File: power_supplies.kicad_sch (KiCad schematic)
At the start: 45 parts, among them IC4 MCP1792T-5002H_CB, IC5 MCP1792T-5002H_CB, J3 12V supply, J5 490107670612, Q3 2N7002BK,215, Q4 Si2333DS, Q5 2N7002BK,215, T1 760390014, U1 PIC10F322-IOT

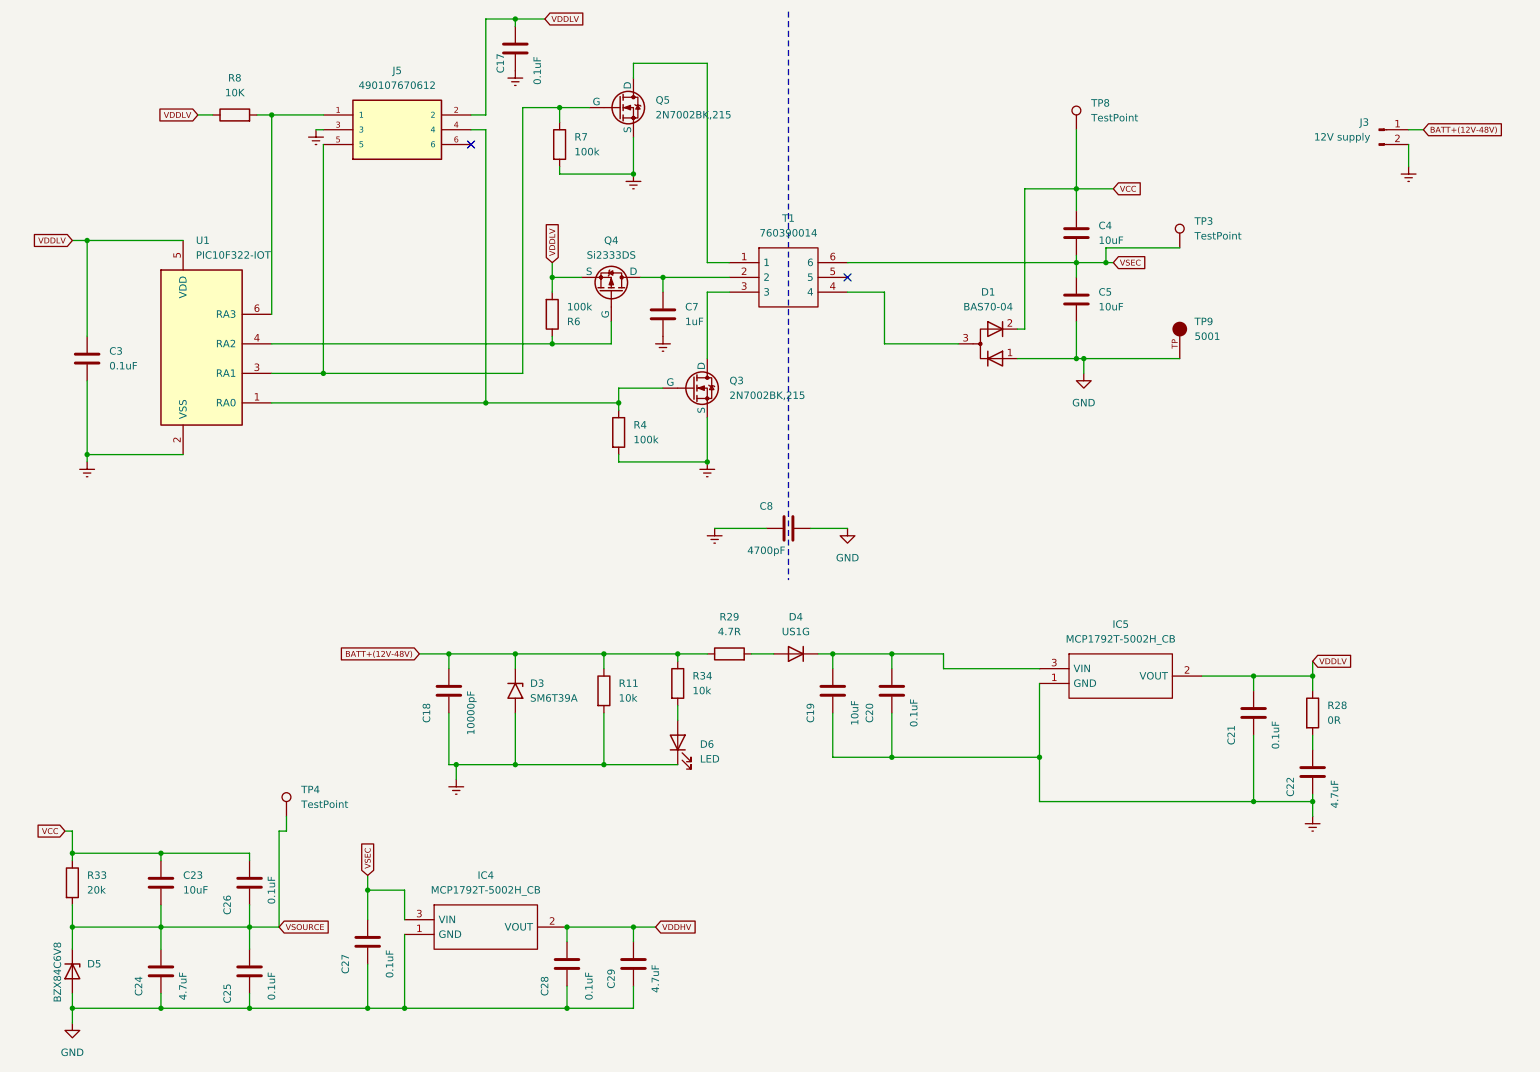
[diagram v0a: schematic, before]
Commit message: Final Design
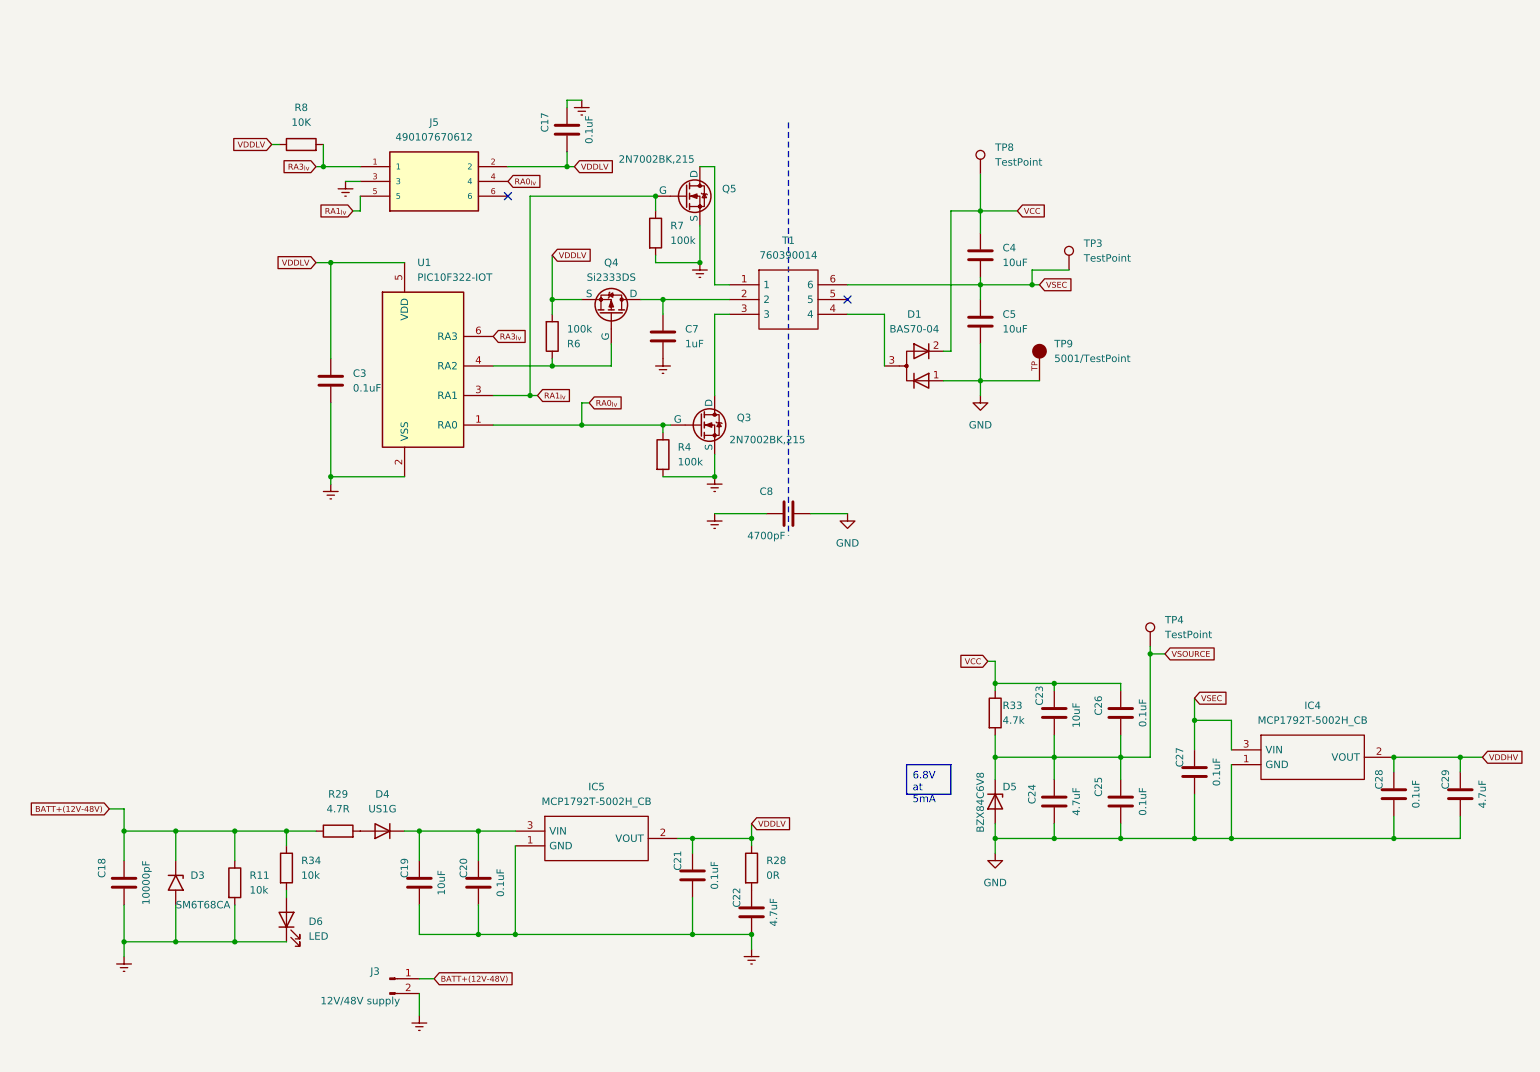
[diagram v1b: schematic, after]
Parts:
- D3: value SM6T39A -> SM6T68CA
- J3: value 12V supply -> 12V/48V supply
- R33: value 20k -> 4.7k
- TP9: value 5001 -> 5001/TestPoint
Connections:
- net Earth: now also C17.2; no longer C17.1
- net VDDLV: now also C17.1; no longer C17.2
- net RA0_{lv}: now reaches J5.4, Q3.1 (G), R4.1, U1.1 (RA0)
- net RA1_{lv}: now reaches J5.5, Q5.1 (G), R7.1, U1.3 (RA1)
- net RA3_{lv}: now reaches J5.1, R8.2, U1.6 (RA3)
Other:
- moved on the sheet: C17, C18, C19, C20, C21, C22, C23, C24, C25, C26, C27, C28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
